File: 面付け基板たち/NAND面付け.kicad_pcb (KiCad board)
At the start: 2 copper layers, 99.1 x 88.9 mm, 105 parts, among them J1 Conn_01x02, J2 Conn_01x02, J3 Conn_01x02

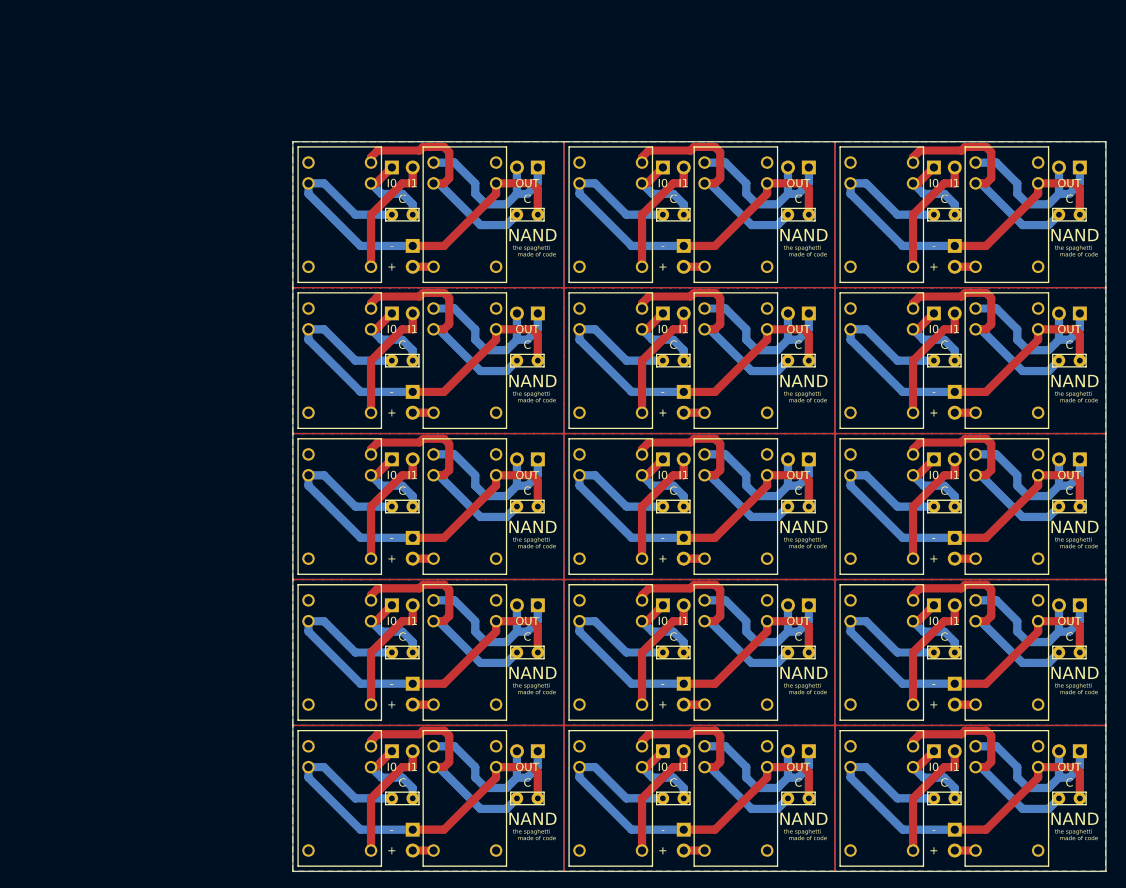
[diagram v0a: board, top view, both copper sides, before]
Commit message: Add files via upload
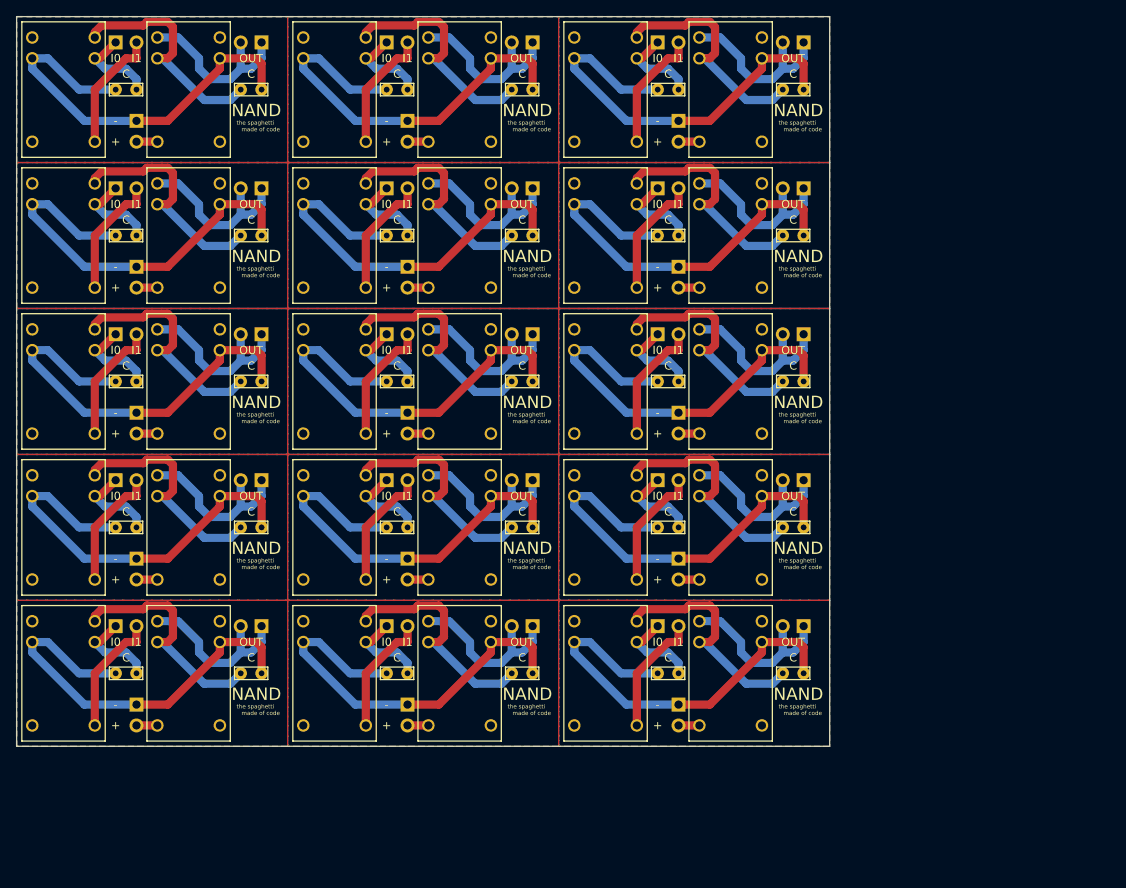
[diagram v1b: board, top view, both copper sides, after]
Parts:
- removed the C1 at (146.1, 130.8)
- removed the C1 at (146.1, 77.5)
- removed the C1 at (113.0, 77.5)
- removed the C1 at (80.0, 77.5)
- removed the C1 at (146.1, 59.7)
- removed the C1 at (113.0, 59.7)
- removed the C1 at (113.0, 130.8)
- removed the C1 at (80.0, 130.8)
- removed the C1 at (146.1, 113.0)
- removed the C1 at (113.0, 113.0)
- removed the C1 at (80.0, 113.0)
- removed the C1 at (146.1, 95.2)
- removed the C1 at (113.0, 95.2)
- removed the C1 at (80.0, 95.2)
- removed the C2 at (161.3, 130.8)
- removed the C2 at (161.3, 77.5)
- removed the C2 at (128.3, 77.5)
- removed the C2 at (95.2, 77.5)
- removed the C2 at (161.3, 59.7)
- removed the C2 at (128.3, 59.7)
- removed the C2 at (128.3, 130.8)
- removed the C2 at (95.2, 130.8)
- removed the C2 at (161.3, 113.0)
- removed the C2 at (128.3, 113.0)
- removed the C2 at (95.2, 113.0)
- removed the C2 at (161.3, 95.2)
- removed the C2 at (128.3, 95.2)
- removed the C2 at (95.2, 95.2)
- removed the J1 at (143.5, 125.1)
- removed the J1 at (143.5, 71.7)
- removed the J1 at (110.5, 71.7)
- removed the J1 at (77.5, 71.7)
- removed the J1 at (143.5, 53.9)
- removed the J1 at (110.5, 53.9)
- removed the J1 at (110.5, 125.1)
- removed the J1 at (77.5, 125.1)
- removed the J1 at (143.5, 107.3)
- removed the J1 at (110.5, 107.3)
- removed the J1 at (77.5, 107.3)
- removed the J1 at (143.5, 89.5)
- removed the J1 at (110.5, 89.5)
- removed the J1 at (77.5, 89.5)
- removed the J2 at (146.1, 134.6)
- removed the J2 at (146.1, 81.3)
- removed the J2 at (113.0, 81.3)
- removed the J2 at (80.0, 81.3)
- removed the J2 at (146.1, 63.5)
- removed the J2 at (113.0, 63.5)
- removed the J2 at (113.0, 134.6)
- removed the J2 at (80.0, 134.6)
- removed the J2 at (146.1, 116.8)
- removed the J2 at (113.0, 116.8)
- removed the J2 at (80.0, 116.8)
- removed the J2 at (146.1, 99.1)
- removed the J2 at (113.0, 99.1)
- removed the J2 at (80.0, 99.1)
- removed the J3 at (161.3, 125.1)
- removed the J3 at (161.3, 71.7)
- removed the J3 at (128.3, 71.7)
- removed the J3 at (95.2, 71.7)
- removed the J3 at (161.3, 53.9)
- removed the J3 at (128.3, 53.9)
- removed the J3 at (128.3, 125.1)
- removed the J3 at (95.2, 125.1)
- removed the J3 at (161.3, 107.3)
- removed the J3 at (128.3, 107.3)
- removed the J3 at (95.2, 107.3)
- removed the J3 at (161.3, 89.5)
- removed the J3 at (128.3, 89.5)
- removed the J3 at (95.2, 89.5)
- removed the SPDT1 at (138.4, 129.5)
- removed the SPDT1 at (138.4, 76.2)
- removed the SPDT1 at (105.4, 76.2)
- removed the SPDT1 at (72.4, 76.2)
- removed the SPDT1 at (138.4, 58.4)
- removed the SPDT1 at (105.4, 58.4)
- removed the SPDT1 at (105.4, 129.5)
- removed the SPDT1 at (72.4, 129.5)
- removed the SPDT1 at (138.4, 111.8)
- removed the SPDT1 at (105.4, 111.8)
- removed the SPDT1 at (72.4, 111.8)
- removed the SPDT1 at (138.4, 94.0)
- removed the SPDT1 at (105.4, 94.0)
- removed the SPDT1 at (72.4, 94.0)
- removed the SPDT2 at (153.7, 129.5)
- removed the SPDT2 at (153.7, 76.2)
- removed the SPDT2 at (120.7, 76.2)
- removed the SPDT2 at (87.6, 76.2)
- removed the SPDT2 at (153.7, 58.4)
- removed the SPDT2 at (120.7, 58.4)
- removed the SPDT2 at (120.7, 129.5)
- removed the SPDT2 at (87.6, 129.5)
- removed the SPDT2 at (153.7, 111.8)
- removed the SPDT2 at (120.7, 111.8)
- removed the SPDT2 at (87.6, 111.8)
- removed the SPDT2 at (153.7, 94.0)
- removed the SPDT2 at (120.7, 94.0)
- removed the SPDT2 at (87.6, 94.0)
- added C1: C, MiyakeFootprintLib:Condensor, F.Cu at (112.4, 115.6)
- added C1: C, MiyakeFootprintLib:Condensor, F.Cu at (112.4, 62.2)
- added C1: C, MiyakeFootprintLib:Condensor, F.Cu at (79.4, 62.2)
- added C1: C, MiyakeFootprintLib:Condensor, F.Cu at (46.4, 62.2)
- added C1: C, MiyakeFootprintLib:Condensor, F.Cu at (112.4, 44.5)
- added C1: C, MiyakeFootprintLib:Condensor, F.Cu at (79.4, 44.5)
- added C1: C, MiyakeFootprintLib:Condensor, F.Cu at (79.4, 115.6)
- added C1: C, MiyakeFootprintLib:Condensor, F.Cu at (46.4, 115.6)
- added C1: C, MiyakeFootprintLib:Condensor, F.Cu at (112.4, 97.8)
- added C1: C, MiyakeFootprintLib:Condensor, F.Cu at (79.4, 97.8)
- added C1: C, MiyakeFootprintLib:Condensor, F.Cu at (46.4, 97.8)
- added C1: C, MiyakeFootprintLib:Condensor, F.Cu at (112.4, 80.0)
- added C1: C, MiyakeFootprintLib:Condensor, F.Cu at (79.4, 80.0)
- added C1: C, MiyakeFootprintLib:Condensor, F.Cu at (46.4, 80.0)
- added C2: C, MiyakeFootprintLib:Condensor, F.Cu at (127.6, 115.6)
- added C2: C, MiyakeFootprintLib:Condensor, F.Cu at (127.6, 62.2)
- added C2: C, MiyakeFootprintLib:Condensor, F.Cu at (94.6, 62.2)
- added C2: C, MiyakeFootprintLib:Condensor, F.Cu at (61.6, 62.2)
- added C2: C, MiyakeFootprintLib:Condensor, F.Cu at (127.6, 44.5)
- added C2: C, MiyakeFootprintLib:Condensor, F.Cu at (94.6, 44.5)
- added C2: C, MiyakeFootprintLib:Condensor, F.Cu at (94.6, 115.6)
- added C2: C, MiyakeFootprintLib:Condensor, F.Cu at (61.6, 115.6)
- added C2: C, MiyakeFootprintLib:Condensor, F.Cu at (127.6, 97.8)
- added C2: C, MiyakeFootprintLib:Condensor, F.Cu at (94.6, 97.8)
- added C2: C, MiyakeFootprintLib:Condensor, F.Cu at (61.6, 97.8)
- added C2: C, MiyakeFootprintLib:Condensor, F.Cu at (127.6, 80.0)
- added C2: C, MiyakeFootprintLib:Condensor, F.Cu at (94.6, 80.0)
- added C2: C, MiyakeFootprintLib:Condensor, F.Cu at (61.6, 80.0)
- added J1: Conn_01x02, Connector_PinHeader_2.54mm:PinHeader_1x02_P2.54mm_Vertical, B.Cu at (109.9, 109.8)
- added J1: Conn_01x02, Connector_PinHeader_2.54mm:PinHeader_1x02_P2.54mm_Vertical, B.Cu at (109.9, 56.5)
- added J1: Conn_01x02, Connector_PinHeader_2.54mm:PinHeader_1x02_P2.54mm_Vertical, B.Cu at (76.8, 56.5)
- added J1: Conn_01x02, Connector_PinHeader_2.54mm:PinHeader_1x02_P2.54mm_Vertical, B.Cu at (43.8, 56.5)
- added J1: Conn_01x02, Connector_PinHeader_2.54mm:PinHeader_1x02_P2.54mm_Vertical, B.Cu at (109.9, 38.7)
- added J1: Conn_01x02, Connector_PinHeader_2.54mm:PinHeader_1x02_P2.54mm_Vertical, B.Cu at (76.8, 38.7)
- added J1: Conn_01x02, Connector_PinHeader_2.54mm:PinHeader_1x02_P2.54mm_Vertical, B.Cu at (76.8, 109.8)
- added J1: Conn_01x02, Connector_PinHeader_2.54mm:PinHeader_1x02_P2.54mm_Vertical, B.Cu at (43.8, 109.8)
- added J1: Conn_01x02, Connector_PinHeader_2.54mm:PinHeader_1x02_P2.54mm_Vertical, B.Cu at (109.9, 92.0)
- added J1: Conn_01x02, Connector_PinHeader_2.54mm:PinHeader_1x02_P2.54mm_Vertical, B.Cu at (76.8, 92.0)
- added J1: Conn_01x02, Connector_PinHeader_2.54mm:PinHeader_1x02_P2.54mm_Vertical, B.Cu at (43.8, 92.0)
- added J1: Conn_01x02, Connector_PinHeader_2.54mm:PinHeader_1x02_P2.54mm_Vertical, B.Cu at (109.9, 74.3)
- added J1: Conn_01x02, Connector_PinHeader_2.54mm:PinHeader_1x02_P2.54mm_Vertical, B.Cu at (76.8, 74.3)
- added J1: Conn_01x02, Connector_PinHeader_2.54mm:PinHeader_1x02_P2.54mm_Vertical, B.Cu at (43.8, 74.3)
- added J2: Conn_01x02, Connector_PinHeader_2.54mm:PinHeader_1x02_P2.54mm_Vertical, B.Cu at (112.4, 119.4)
- added J2: Conn_01x02, Connector_PinHeader_2.54mm:PinHeader_1x02_P2.54mm_Vertical, B.Cu at (112.4, 66.0)
- added J2: Conn_01x02, Connector_PinHeader_2.54mm:PinHeader_1x02_P2.54mm_Vertical, B.Cu at (79.4, 66.0)
- added J2: Conn_01x02, Connector_PinHeader_2.54mm:PinHeader_1x02_P2.54mm_Vertical, B.Cu at (46.4, 66.0)
- added J2: Conn_01x02, Connector_PinHeader_2.54mm:PinHeader_1x02_P2.54mm_Vertical, B.Cu at (112.4, 48.3)
- added J2: Conn_01x02, Connector_PinHeader_2.54mm:PinHeader_1x02_P2.54mm_Vertical, B.Cu at (79.4, 48.3)
- added J2: Conn_01x02, Connector_PinHeader_2.54mm:PinHeader_1x02_P2.54mm_Vertical, B.Cu at (79.4, 119.4)
- added J2: Conn_01x02, Connector_PinHeader_2.54mm:PinHeader_1x02_P2.54mm_Vertical, B.Cu at (46.4, 119.4)
- added J2: Conn_01x02, Connector_PinHeader_2.54mm:PinHeader_1x02_P2.54mm_Vertical, B.Cu at (112.4, 101.6)
- added J2: Conn_01x02, Connector_PinHeader_2.54mm:PinHeader_1x02_P2.54mm_Vertical, B.Cu at (79.4, 101.6)
- added J2: Conn_01x02, Connector_PinHeader_2.54mm:PinHeader_1x02_P2.54mm_Vertical, B.Cu at (46.4, 101.6)
- added J2: Conn_01x02, Connector_PinHeader_2.54mm:PinHeader_1x02_P2.54mm_Vertical, B.Cu at (112.4, 83.8)
- added J2: Conn_01x02, Connector_PinHeader_2.54mm:PinHeader_1x02_P2.54mm_Vertical, B.Cu at (79.4, 83.8)
- added J2: Conn_01x02, Connector_PinHeader_2.54mm:PinHeader_1x02_P2.54mm_Vertical, B.Cu at (46.4, 83.8)
- added J3: Conn_01x02, Connector_PinHeader_2.54mm:PinHeader_1x02_P2.54mm_Vertical, B.Cu at (127.6, 109.8)
- added J3: Conn_01x02, Connector_PinHeader_2.54mm:PinHeader_1x02_P2.54mm_Vertical, B.Cu at (127.6, 56.5)
- added J3: Conn_01x02, Connector_PinHeader_2.54mm:PinHeader_1x02_P2.54mm_Vertical, B.Cu at (94.6, 56.5)
- added J3: Conn_01x02, Connector_PinHeader_2.54mm:PinHeader_1x02_P2.54mm_Vertical, B.Cu at (61.6, 56.5)
- added J3: Conn_01x02, Connector_PinHeader_2.54mm:PinHeader_1x02_P2.54mm_Vertical, B.Cu at (127.6, 38.7)
- added J3: Conn_01x02, Connector_PinHeader_2.54mm:PinHeader_1x02_P2.54mm_Vertical, B.Cu at (94.6, 38.7)
- added J3: Conn_01x02, Connector_PinHeader_2.54mm:PinHeader_1x02_P2.54mm_Vertical, B.Cu at (94.6, 109.8)
- added J3: Conn_01x02, Connector_PinHeader_2.54mm:PinHeader_1x02_P2.54mm_Vertical, B.Cu at (61.6, 109.8)
- added J3: Conn_01x02, Connector_PinHeader_2.54mm:PinHeader_1x02_P2.54mm_Vertical, B.Cu at (127.6, 92.0)
- added J3: Conn_01x02, Connector_PinHeader_2.54mm:PinHeader_1x02_P2.54mm_Vertical, B.Cu at (94.6, 92.0)
- added J3: Conn_01x02, Connector_PinHeader_2.54mm:PinHeader_1x02_P2.54mm_Vertical, B.Cu at (61.6, 92.0)
- added J3: Conn_01x02, Connector_PinHeader_2.54mm:PinHeader_1x02_P2.54mm_Vertical, B.Cu at (127.6, 74.3)
- added J3: Conn_01x02, Connector_PinHeader_2.54mm:PinHeader_1x02_P2.54mm_Vertical, B.Cu at (94.6, 74.3)
- added J3: Conn_01x02, Connector_PinHeader_2.54mm:PinHeader_1x02_P2.54mm_Vertical, B.Cu at (61.6, 74.3)
- added SPDT1: 946H-1C-24D, MiyakeFootprintLib:946H-1C-24D, F.Cu at (104.8, 114.3)
- added SPDT1: 946H-1C-24D, MiyakeFootprintLib:946H-1C-24D, F.Cu at (104.8, 61.0)
- added SPDT1: 946H-1C-24D, MiyakeFootprintLib:946H-1C-24D, F.Cu at (71.8, 61.0)
- added SPDT1: 946H-1C-24D, MiyakeFootprintLib:946H-1C-24D, F.Cu at (38.7, 61.0)
- added SPDT1: 946H-1C-24D, MiyakeFootprintLib:946H-1C-24D, F.Cu at (104.8, 43.2)
- added SPDT1: 946H-1C-24D, MiyakeFootprintLib:946H-1C-24D, F.Cu at (71.8, 43.2)
- added SPDT1: 946H-1C-24D, MiyakeFootprintLib:946H-1C-24D, F.Cu at (71.8, 114.3)
- added SPDT1: 946H-1C-24D, MiyakeFootprintLib:946H-1C-24D, F.Cu at (38.7, 114.3)
- added SPDT1: 946H-1C-24D, MiyakeFootprintLib:946H-1C-24D, F.Cu at (104.8, 96.5)
- added SPDT1: 946H-1C-24D, MiyakeFootprintLib:946H-1C-24D, F.Cu at (71.8, 96.5)
- added SPDT1: 946H-1C-24D, MiyakeFootprintLib:946H-1C-24D, F.Cu at (38.7, 96.5)
- added SPDT1: 946H-1C-24D, MiyakeFootprintLib:946H-1C-24D, F.Cu at (104.8, 78.7)
- added SPDT1: 946H-1C-24D, MiyakeFootprintLib:946H-1C-24D, F.Cu at (71.8, 78.7)
- added SPDT1: 946H-1C-24D, MiyakeFootprintLib:946H-1C-24D, F.Cu at (38.7, 78.7)
- added SPDT2: 946H-1C-24D, MiyakeFootprintLib:946H-1C-24D, F.Cu at (120.0, 114.3)
- added SPDT2: 946H-1C-24D, MiyakeFootprintLib:946H-1C-24D, F.Cu at (120.0, 61.0)
- added SPDT2: 946H-1C-24D, MiyakeFootprintLib:946H-1C-24D, F.Cu at (87.0, 61.0)
- added SPDT2: 946H-1C-24D, MiyakeFootprintLib:946H-1C-24D, F.Cu at (54.0, 61.0)
- added SPDT2: 946H-1C-24D, MiyakeFootprintLib:946H-1C-24D, F.Cu at (120.0, 43.2)
- added SPDT2: 946H-1C-24D, MiyakeFootprintLib:946H-1C-24D, F.Cu at (87.0, 43.2)
- added SPDT2: 946H-1C-24D, MiyakeFootprintLib:946H-1C-24D, F.Cu at (87.0, 114.3)
- added SPDT2: 946H-1C-24D, MiyakeFootprintLib:946H-1C-24D, F.Cu at (54.0, 114.3)
- added SPDT2: 946H-1C-24D, MiyakeFootprintLib:946H-1C-24D, F.Cu at (120.0, 96.5)
- added SPDT2: 946H-1C-24D, MiyakeFootprintLib:946H-1C-24D, F.Cu at (87.0, 96.5)
- added SPDT2: 946H-1C-24D, MiyakeFootprintLib:946H-1C-24D, F.Cu at (54.0, 96.5)
- added SPDT2: 946H-1C-24D, MiyakeFootprintLib:946H-1C-24D, F.Cu at (120.0, 78.7)
- added SPDT2: 946H-1C-24D, MiyakeFootprintLib:946H-1C-24D, F.Cu at (87.0, 78.7)
- added SPDT2: 946H-1C-24D, MiyakeFootprintLib:946H-1C-24D, F.Cu at (54.0, 78.7)
- moved J2 36.9 mm to (46.4, 48.3)
- moved C1 36.9 mm to (46.4, 44.5)
- moved C2 36.9 mm to (61.6, 44.5)
- moved J1 36.9 mm to (43.8, 38.7)
- moved J3 36.9 mm to (61.6, 38.7)
- moved SPDT1 36.9 mm to (38.7, 43.2)
- moved SPDT2 36.9 mm to (54.0, 43.2)
